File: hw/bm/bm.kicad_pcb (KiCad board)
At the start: 2 copper layers, 159 x 47.5 mm, 51 parts, among them P1 PX0707/06S, P2 PX0707/06S, P3 XT60 Male, P4 XT60 Male, P5 JST-XH, P6 JST-XH, P7 I²C, P8 I²C, U1 MCP3428, U2 MCP3428

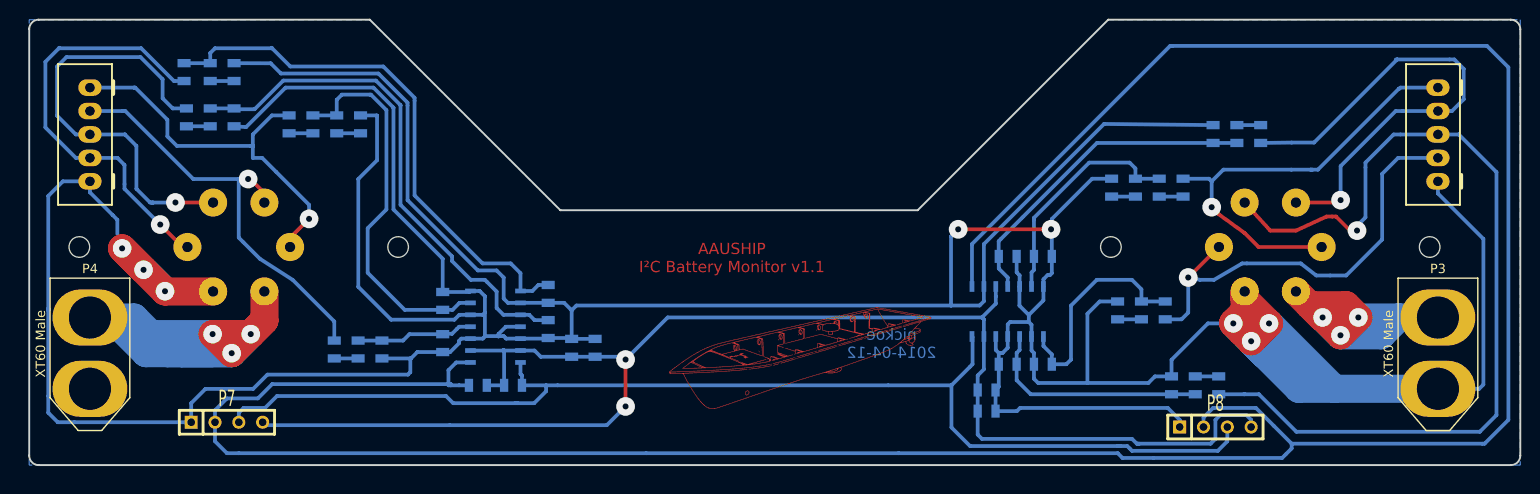
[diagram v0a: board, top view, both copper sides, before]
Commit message: Update bm
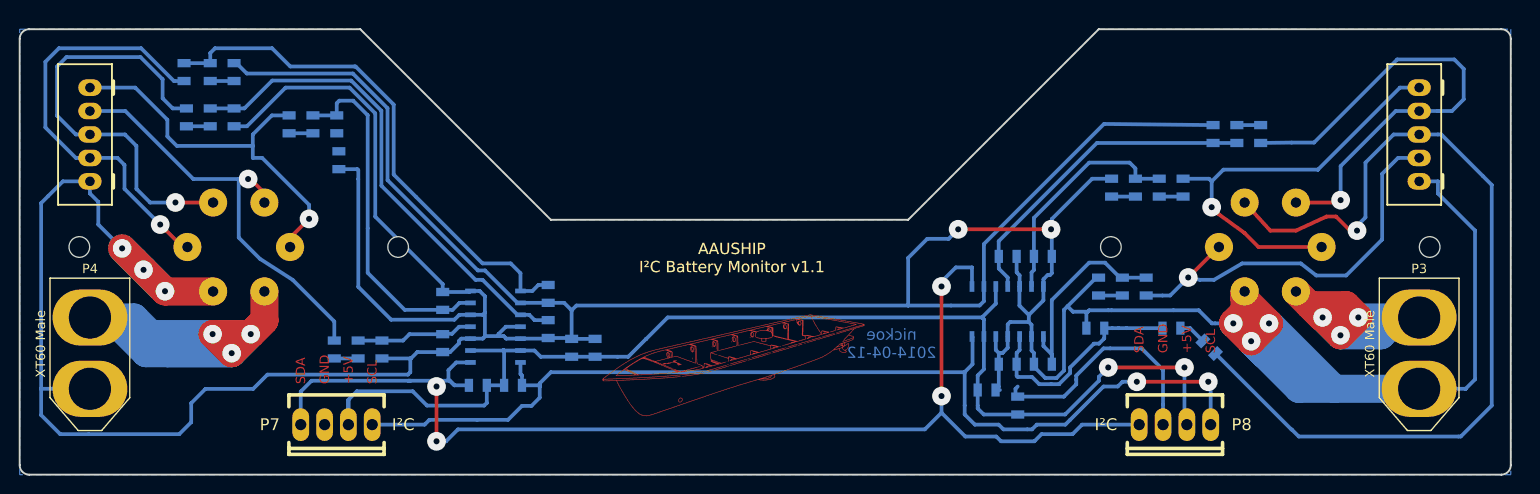
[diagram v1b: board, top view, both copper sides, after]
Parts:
- P7, P8: footprint Connect:SIL-4 -> argo:Socket_MOLEX-KK-RM2-54mm_Lock_4pin_straight
- moved P7 11.7 mm to (90.4, 121.9), turned to 180 degrees
- moved R17 10.2 mm to (171.3, 111.6), turned to 180 degrees
- moved VAL 7.15 mm to (132.8, 115.6)
- moved R8 6.60 mm to (179.5, 111.6), turned to 180 degrees
- moved R26 4.47 mm to (90.7, 93.7), turned to 270 degrees
- moved P8 4.33 mm to (179.8, 121.9), turned to 180 degrees
- moved R1 4.19 mm to (183.5, 113.7), turned to 135 degrees
- moved C4 3.37 mm to (163.1, 119.9), turned to 90 degrees
- moved R12 3.25 mm to (171.7, 107.2)
- moved R4 3.25 mm to (176.8, 107.2)
- moved R11 3.25 mm to (174.2, 107.2)
- moved P3 2.00 mm to (205.9, 114.3)
- moved P5 2.00 mm to (205.9, 91.0)
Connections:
- P7 pad 1: GND -> Net-(P7-Pad1)
- P7 pad 2: N-0000015 -> +5V
- P7 pad 3: N-0000016 -> GND
- P7 pad 4: +5V -> Net-(P7-Pad4)
- P8 pad 1: GND -> Net-(P7-Pad1)
- P8 pad 2: N-0000015 -> +5V
- P8 pad 3: N-0000016 -> GND
- P8 pad 4: +5V -> Net-(P7-Pad4)
- R33 pad 2: N-0000015 -> Net-(P7-Pad4)
- R35 pad 1: N-0000016 -> Net-(P7-Pad1)
- U1 pad 7: N-0000016 -> Net-(P7-Pad1)
- U1 pad 8: N-0000015 -> Net-(P7-Pad4)
- U2 pad 7: N-0000016 -> Net-(P7-Pad1)
- U2 pad 8: N-0000015 -> Net-(P7-Pad4)
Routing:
- net N-0000015: track 298.3 -> 0.00 mm
- net Net-(P7-Pad4): track 0.00 -> 131.0 mm, vias 0 -> 4
- net N-0000016: track 127.6 -> 0.00 mm
- net Net-(P7-Pad1): track 0.00 -> 113.0 mm, vias 0 -> 2
- net +5V: track 157.1 -> 129.6 mm
- net Net-(C12-Pad1): track 41.5 -> 37.6 mm
- net Net-(P2-Pad6): track 64.6 -> 61.3 mm
- net Net-(P1-Pad2): track 48.0 -> 44.8 mm
- net Net-(C8-Pad1): track 55.4 -> 52.5 mm
- net Net-(R25-Pad2): track 2.54 -> 0.00 mm
- net Net-(P1-Pad5): track 47.7 -> 45.5 mm
- net Net-(C6-Pad1): track 58.4 -> 56.6 mm
- net Net-(C5-Pad1): track 24.2 -> 22.6 mm
- net GND: track 556.8 -> 558.5 mm
- net Net-(P1-Pad4): track 54.1 -> 53.6 mm
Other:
- board text added: "+5V"
- board text added: "GND"
- board text added: "SCL"
- board text added: "SDA"
- board text added: "TODO ---- * Buccaneer connectors has to match up with the charge plug, the socket and plug has mirrored numbering * Componets has to be free of the buccaneer connectors"
- board text removed: "TODO ---- * Deans connectors has to be replaces with XT60 compatible footprints * Buccaneer connectors has to match up with the charge plug, the socket and plug has mirrored numbering * Componets has to be free of the buccaneer connectors"
